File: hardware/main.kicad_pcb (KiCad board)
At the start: 2 copper layers, 84.6 x 84.6 mm, 133 parts, among them J1 USB_DEBUG, J2 USB_TO_ANDROID, M1 Mounting Hole, M2 Mounting Hole, M3 Mounting Hole, M4 Mounting Hole, P1 VBAT-TEST, P10 ANDROID-SERIAL-TEST, P11 MOTOR-R, P12 MOTOR-L, P13 AND5V, P14 AUX, P15 MOTOR-PWM-TEST, P2 USB-VBUS, P3 SERVO-TILT, P4 JTAG10, P5 POWER-CHARGE, P6 POWER, P7 BATCHG, P8 12VIN, P9 BAT, Q1 ZXMP2120FFTA, Q2 BD242CG, Q3 IRLML2803TRPBF, Q4 IRLML2803TRPBF, U1 STM32F102C6, U2 BQ24450, U3 ZLDO1117, U4 AP6502, U5 7408, U6 MC33926, U7 MC33926, U8 FT312D, X1 8MHz, X2 12MHz

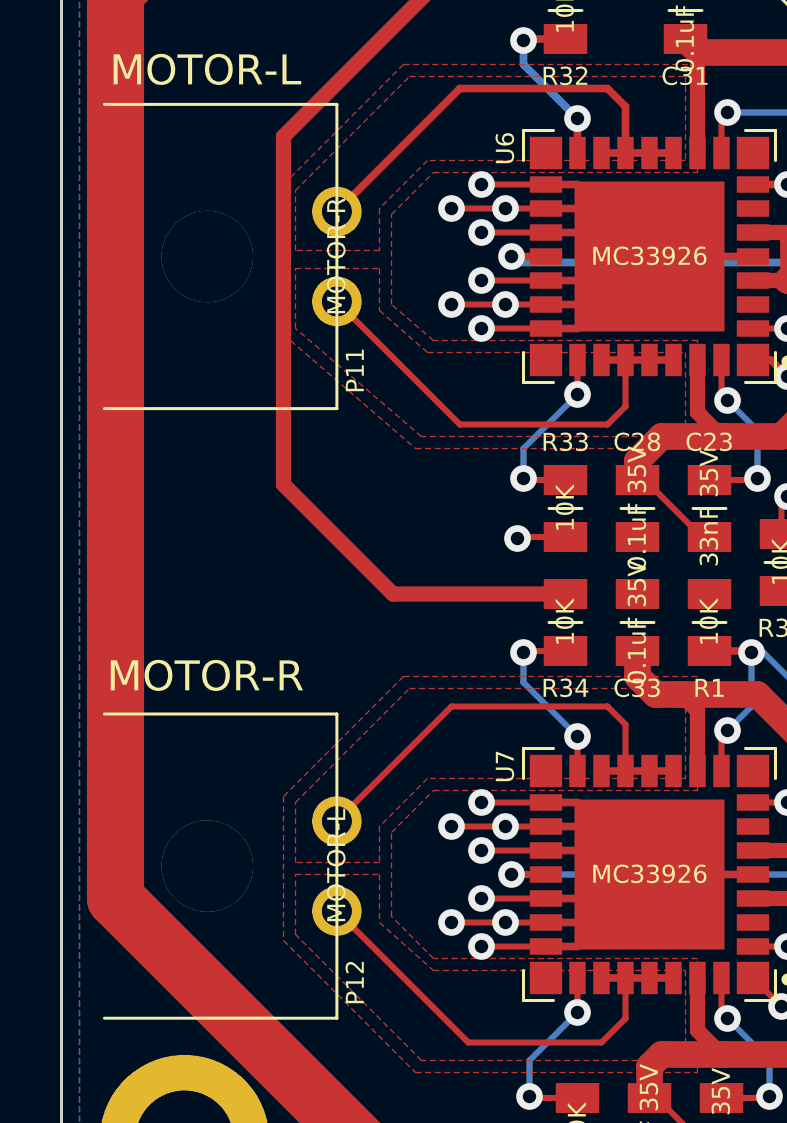
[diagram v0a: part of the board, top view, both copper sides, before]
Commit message: working
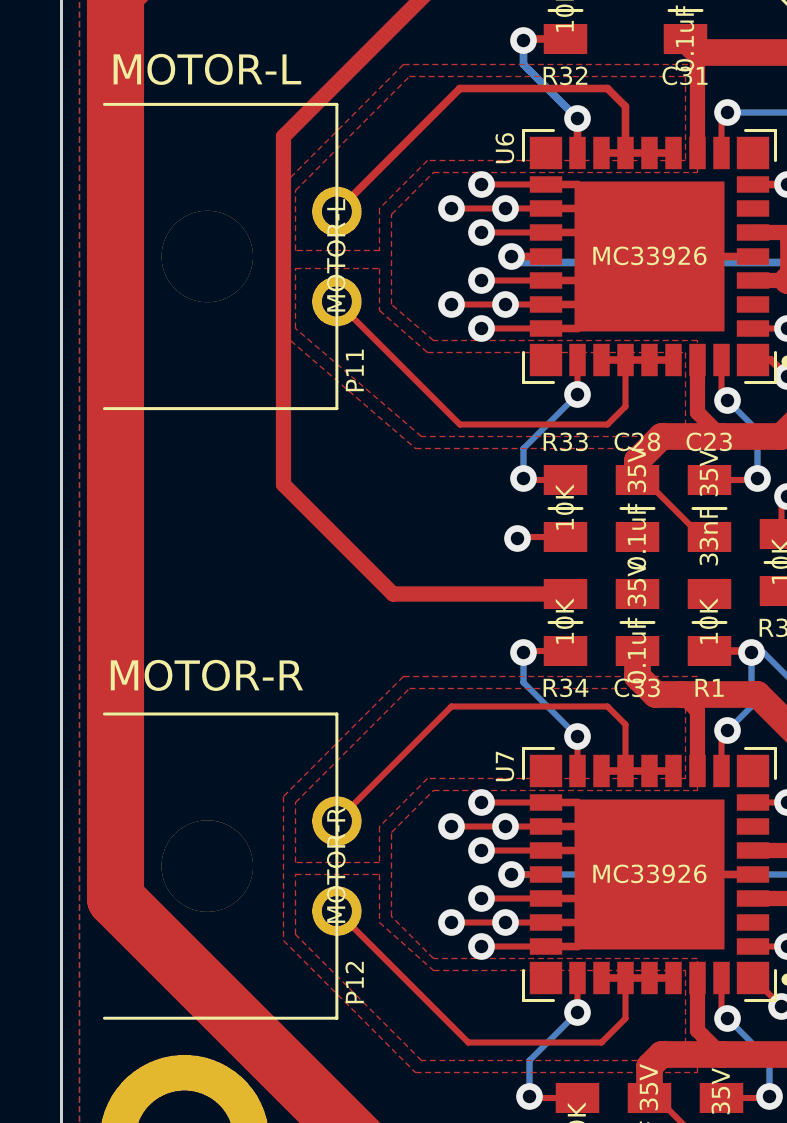
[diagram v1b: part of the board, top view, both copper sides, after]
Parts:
- P11: value MOTOR-R -> MOTOR-L
- P12: value MOTOR-L -> MOTOR-R
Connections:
- P15 pad 1: /Motor Controllers/MOTOR-L-PWM -> /Motor Controllers/MOTOR-R-PWM
- P15 pad 2: /Motor Controllers/MOTOR-R-PWM -> /Motor Controllers/MOTOR-L-PWM
- Q3 pad 1: /Motor Controllers/MOTOR-R-DIR -> /Motor Controllers/MOTOR-L-DIR
- Q4 pad 1: /Motor Controllers/MOTOR-L-DIR -> /Motor Controllers/MOTOR-R-DIR
- R10 pad 2: /Motor Controllers/MOTOR-R-DIR -> /Motor Controllers/MOTOR-L-DIR
- R11 pad 2: /Motor Controllers/MOTOR-L-DIR -> /Motor Controllers/MOTOR-R-DIR
- R26 pad 1: /Motor Controllers/MOTOR-R-DIR -> /Motor Controllers/MOTOR-L-DIR
- R27 pad 1: /Motor Controllers/MOTOR-L-DIR -> /Motor Controllers/MOTOR-R-DIR
- R30 pad 1: /Motor Controllers/MOTOR-R-PWM -> /Motor Controllers/MOTOR-L-PWM
- R31 pad 1: /Motor Controllers/MOTOR-L-PWM -> /Motor Controllers/MOTOR-R-PWM
- U1 pad 12: /Motor Controllers/MOTOR-L-PWM -> /Motor Controllers/MOTOR-R-PWM
- U1 pad 13: /Motor Controllers/MOTOR-R-PWM -> /Motor Controllers/MOTOR-L-PWM
- U5 pad 1: /Motor Controllers/MOTOR-R-PWM -> /Motor Controllers/MOTOR-L-PWM
- U5 pad 10: /Motor Controllers/MOTOR-L-DIR -> /Motor Controllers/MOTOR-R-DIR
- U5 pad 12: /Motor Controllers/MOTOR-L-PWM -> /Motor Controllers/MOTOR-R-PWM
- U5 pad 2: /Motor Controllers/MOTOR-R-DIR -> /Motor Controllers/MOTOR-L-DIR
- U5 pad 4: /Motor Controllers/MOTOR-R-PWM -> /Motor Controllers/MOTOR-L-PWM
- U5 pad 9: /Motor Controllers/MOTOR-L-PWM -> /Motor Controllers/MOTOR-R-PWM
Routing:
- net /Motor Controllers/MOTOR-R-PWM: track 69.0 -> 56.5 mm, vias 4 -> 2
- net /Motor Controllers/MOTOR-L-PWM: track 56.5 -> 69.0 mm, vias 2 -> 4
- net /Motor Controllers/MOTOR-R-DIR: track 31.9 -> 21.1 mm, vias 2 -> 0
- net /Motor Controllers/MOTOR-L-DIR: track 21.1 -> 31.9 mm, vias 0 -> 2
